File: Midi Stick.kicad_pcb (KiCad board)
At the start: 2 copper layers, 47.1 x 17.5 mm, 56 parts, among them J2 Aux, J3 ICSP, J8 USB_C_Receptacle_USB2.0_16P, Q1 Mosfet N, SW1 SW_Push, U1 W25Q128JVS, U2 NCP1117-3.3_SOT223, U3 RP2350_60QFN, Y1 ABM8-272-T3

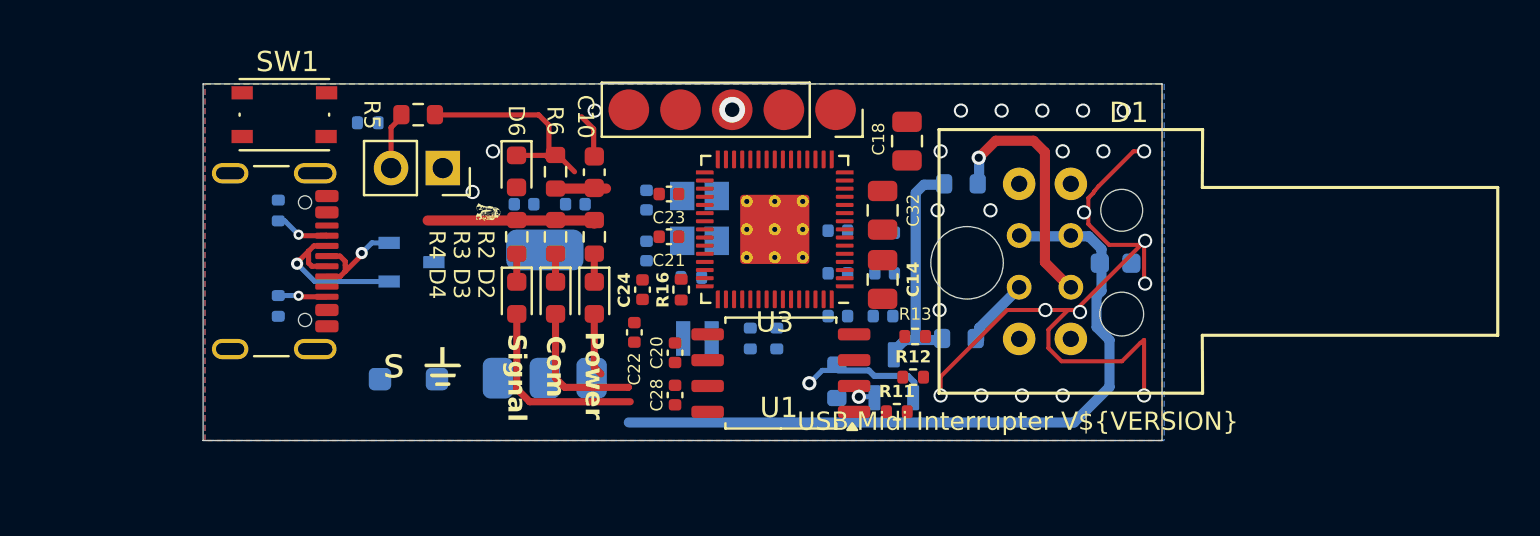
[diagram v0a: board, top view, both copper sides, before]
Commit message: single sided
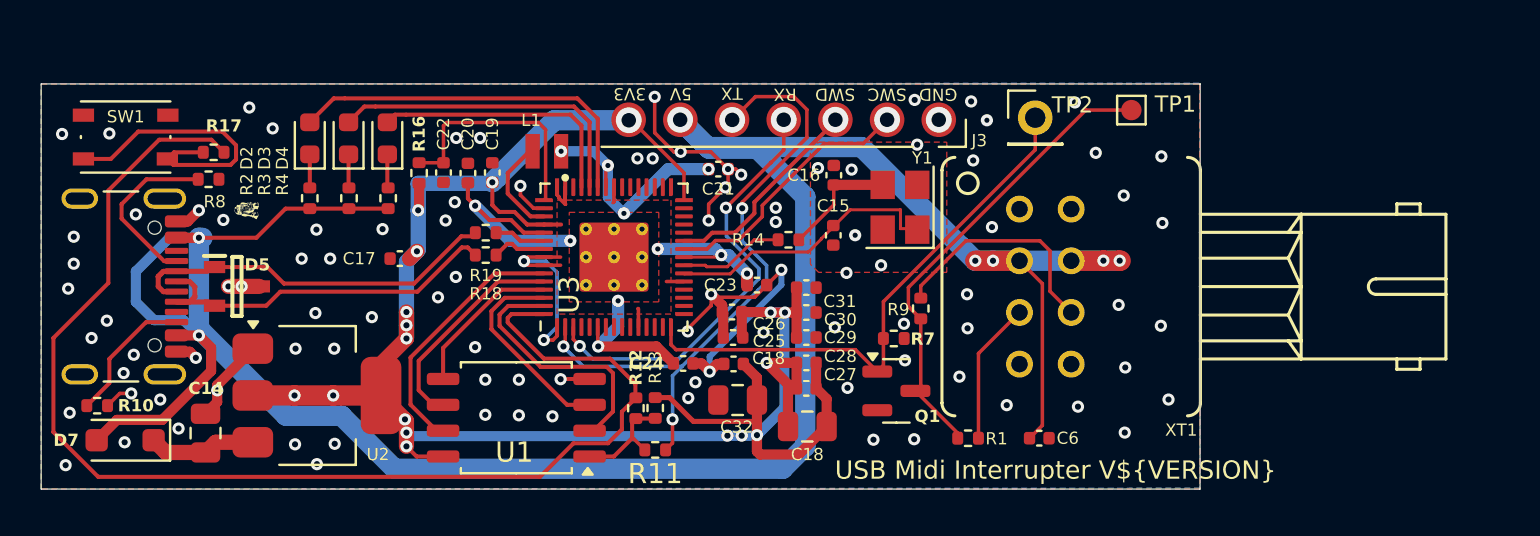
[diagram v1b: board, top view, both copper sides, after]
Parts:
- removed C10: 1uF, Capacitor_SMD:C_0603_1608Metric
- removed D1: HFBR-141X, Midi Stick:HFBR-x41xZ
- removed D6: TVS Diode, Diode_SMD:D_0603_1608Metric
- removed J2: Aux, Connector_PinSocket_2.54mm:PinSocket_1x02_P2.54mm_Vertical
- removed R5: 470ohm, Resistor_SMD:R_0603_1608Metric
- removed R6: 10k, Resistor_SMD:R_0603_1608Metric
- added C18: 100n, Capacitor_SMD:C_0402_1005Metric, F.Cu at (110.0, 67.5)
- added TP1: Out Sense, TestPoint:TestPoint_Pad_1.0x1.0mm, F.Cu at (129.5, 55.0)
- added TP2: Out, Connector_PinHeader_2.54mm:PinHeader_1x01_P2.54mm_Vertical, F.Cu at (124.8, 55.4)
- added XT1: HFBR-1412, Midi Stick:HFBR-X41X, F.Cu at (126.6, 63.7)
- C15, C16, C17, C19, C25, C26, C27, C29, C30, C31, D5, D7, L1, R10, R14, R17, R18, R19, R8, U2, Y1: moved to F.Cu
- C6: value 100nF -> 100n; footprint Capacitor_SMD:C_0603_1608Metric -> Capacitor_SMD:C_0402_1005Metric; moved to F.Cu
- J3: footprint Connector_PinSocket_2.54mm:PinSocket_1x05_P2.54mm_Vertical -> Connector_PinSocket_2.54mm:PinSocket_1x07_P2.54mm_Vertical
- Q1: value Mosfet N -> T2N7002AK; footprint Midi Stick:SOT95P237X112-3N -> Package_TO_SOT_SMD:SOT-23; moved to F.Cu
- R1: value 47Ohm -> 470; footprint Resistor_SMD:R_0603_1608Metric -> Resistor_SMD:R_0402_1005Metric; moved to F.Cu
- R2, R3, R4: footprint Resistor_SMD:R_0603_1608Metric -> Resistor_SMD:R_0402_1005Metric
- R7: footprint Resistor_SMD:R_0603_1608Metric -> Resistor_SMD:R_0402_1005Metric; moved to F.Cu
- R9: value 150Ohm -> 150; footprint Resistor_SMD:R_0603_1608Metric -> Resistor_SMD:R_0402_1005Metric; moved to F.Cu
- moved C14 34.1 mm to (84.0, 70.9), turned to 90 degrees
- moved D2 16.0 mm to (89.1, 56.4), turned to 90 degrees
- moved R18 14.9 mm to (97.8, 62.2), turned to 0 degrees
- moved C18 14.9 mm to (113.6, 70.6), turned to 180 degrees
- moved D7 14.2 mm to (80.1, 71.3)
- moved R2 14.1 mm to (89.1, 59.4)
- moved R16 14.1 mm to (94.5, 58.1), turned to 90 degrees
- moved R19 14.0 mm to (97.8, 61.1), turned to 0 degrees
- moved R12 13.7 mm to (105.2, 69.7), turned to -90 degrees
- moved C20 13.5 mm to (96.9, 58.1), turned to 90 degrees
- moved R13 13.2 mm to (106.1, 69.7), turned to -90 degrees
- moved U1 13.2 mm to (99.3, 70.1)
- moved D3 12.8 mm to (91.0, 56.4), turned to 90 degrees
- moved C22 12.2 mm to (95.7, 58.1)
- moved R11 12.0 mm to (106.1, 71.7)
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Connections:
- C14 pad 1: VBUS -> Net-(D7-K)
- C6 pad 1: GND -> VBUS
- C6 pad 2: VBUS -> GND
- D7 pad 1: VBUS -> Net-(D7-K)
- D7 pad 2: Net-(D7-A) -> VBUS
- J3 pad 1: /SWCLK -> GND
- J3 pad 2: GND -> /SWCLK
- J3 pad 4: GND -> /UART0 RX
- J3 pad 5: +3V3 -> /UART0 TX
- J8 pad A4: Net-(D7-A) -> VBUS
- J8 pad A9: Net-(D7-A) -> VBUS
- J8 pad B4: Net-(D7-A) -> VBUS
- J8 pad B9: Net-(D7-A) -> VBUS
- Q1 pad 1: (no net) -> /Out
- Q1 pad 2: (no net) -> GND
- Q1 pad 3: (no net) -> /Out Sense
- R1 pad 1: /Out Sense -> Net-(R1-Pad1)
- R1 pad 2: Net-(D1-PadCH) -> /Out Sense
- R11 pad 1: /GPIO0 -> /UART0 TX
- R2 pad 1: Net-(D2-Pad1) -> VBUS
- R2 pad 2: VBUS -> Net-(D2-Pad1)
- R3 pad 1: Net-(D3-Pad1) -> VBUS
- R3 pad 2: VBUS -> Net-(D3-Pad1)
- R4 pad 1: Net-(D4-Pad1) -> VBUS
- R4 pad 2: VBUS -> Net-(D4-Pad1)
- R7 pad 1: GND -> /Out
- R7 pad 2: /Out -> GND
- R9 pad 1: /Out Sense -> Net-(R9-Pad1)
- R9 pad 2: Net-(D1-PadCE) -> /Out Sense
- U2 pad 3: VBUS -> Net-(D7-K)
- U3 pad 15: unconnected-(U3-GPIO11-Pad15) -> /Out
- U3 pad 2: unconnected-(U3-GPIO0-Pad2) -> /UART0 TX
- U3 pad 27: /Power LED -> unconnected-(U3-GPIO16-Pad27)
- U3 pad 28: /Com LED -> unconnected-(U3-GPIO17-Pad28)
- U3 pad 29: /Signal LED -> unconnected-(U3-GPIO18-Pad29)
- U3 pad 3: unconnected-(U3-GPIO1-Pad3) -> /UART0 RX
- U3 pad 37: /Out -> unconnected-(U3-GPIO25-Pad37)
- U3 pad 40: unconnected-(U3-GPIO26_ADC0-Pad40) -> /Power LED
- U3 pad 41: unconnected-(U3-GPIO27_ADC1-Pad41) -> /Com LED
- U3 pad 42: unconnected-(U3-GPIO28_ADC2-Pad42) -> /Signal LED
- U3 pad 8: /Aux -> unconnected-(U3-GPIO5-Pad8)
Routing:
- net +3V3: track 0.38 -> 113.7 mm, vias 0 -> 19
- net VBUS: track 44.2 -> 126.6 mm, vias 0 -> 7
- net /QSPI_SS: track 0.00 -> 61.9 mm
- net +1V1: track 0.00 -> 37.0 mm, vias 0 -> 11
- net /UART0 TX: track 0.00 -> 32.2 mm, vias 0 -> 4
- net /UART0 RX: track 0.00 -> 21.6 mm, vias 0 -> 3
- net /Out: track 6.37 -> 27.2 mm, vias 1 -> 0
- net /Power LED: track 3.22 -> 18.4 mm
- net /~{USB_BOOT}: track 0.00 -> 14.5 mm
- net /XIN: track 0.00 -> 13.7 mm
- net /USB_D+: track 5.30 -> 18.2 mm, vias 1 -> 0
- net Net-(D1-PadCE): track 12.7 -> 0.00 mm, vias 1 -> 0
- net /QSPI_SD3: track 0.00 -> 12.7 mm
- net /SWCLK: track 0.41 -> 12.9 mm, vias 0 -> 1
- net /QSPI_SD1: track 0.83 -> 12.9 mm, vias 1 -> 0
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- added copper zone on F.Cu, net +1V1
- added copper zone on F.Cu, net +3V3
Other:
- board size 47.1 x 17.5 mm -> 57 x 19.9 mm
- board text added: "3V3"
- board text added: "5V"
- board text added: "GND"
- board text added: "RX"
- board text added: "SWC"
- board text added: "SWD"
- board text added: "TX"
- board text removed: "Com"
- board text removed: "Power"
- board text removed: "Signal"
- board text removed: "for HFBR"
- board text removed: "for IF E96E"
- board text removed: "s"
